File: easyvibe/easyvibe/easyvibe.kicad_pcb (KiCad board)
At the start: 2 copper layers, 111 x 54.6 mm, 80 parts, among them U1 TL062, U2 TL062, U3 TL062, U4 TL062

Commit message: some fixes
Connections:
- C2 pad 2: Net-(U1B--) -> Net-(U1B-+)
- C3 pad 2: Net-(U2B--) -> Net-(U2B-+)
- C4 pad 2: Net-(U3B--) -> Net-(U3B-+)
- C5 pad 2: Net-(U4B--) -> Net-(U4B-+)
- C6 pad 1: Net-(J_STOMP5-Pin_1) -> Net-(C6-Pad1)
- C6 pad 2: Net-(C6-Pad2) -> Net-(J_STOMP5-Pin_1)
- C8 pad 1: Net-(C8-Pad1) -> Net-(J_RATE1-Pin_1)
- LDR1 pad 1: Net-(U1B--) -> Net-(U1B-+)
- LDR2 pad 1: Net-(U2B--) -> Net-(U2B-+)
- LDR3 pad 1: Net-(U3B--) -> Net-(U3B-+)
- LDR4 pad 1: Net-(U4B--) -> Net-(U4B-+)
- R10 pad 1: Net-(U3B-+) -> Net-(U3B--)
- R11 pad 2: Net-(U4B-+) -> Net-(U4B--)
- R12 pad 1: Net-(U4B-+) -> Net-(U4B--)
- R13 pad 1: Net-(C6-Pad2) -> Net-(C6-Pad1)
- R14 pad 2: Net-(C6-Pad2) -> Net-(C6-Pad1)
- R20 pad 2: Net-(C8-Pad1) -> Net-(J_RATE1-Pin_1)
- R5 pad 2: Net-(U1B-+) -> Net-(U1B--)
- R6 pad 1: Net-(U1B-+) -> Net-(U1B--)
- R7 pad 2: Net-(U2B-+) -> Net-(U2B--)
- R8 pad 1: Net-(U2B-+) -> Net-(U2B--)
- R9 pad 2: Net-(U3B-+) -> Net-(U3B--)
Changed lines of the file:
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@@
 			(layers "*.Cu" "*.Mask")
 			(remove_unused_layers no)
-			(net "Net-(U3B-+)")
+			(net "Net-(U3B--)")
 			(pintype "passive")
 		)
@@
 			(layers "*.Cu" "*.Mask")
 			(remove_unused_layers no)
-			(net "Net-(U4B--)")
+			(net "Net-(U4B-+)")
 			(pintype "passive")
 		)
@@
 			(layers "*.Cu" "*.Mask")
 			(remove_unused_layers no)
-			(net "Net-(C8-Pad1)")
+			(net "Net-(J_RATE1-Pin_1)")
 			(pintype "passive")
 		)
@@
 			(layers "*.Cu" "*.Mask")
 			(remove_unused_layers no)
-			(net "Net-(U1B-+)")
+			(net "Net-(U1B--)")
 			(pintype "passive")
 		)
@@
 			(layers "*.Cu" "*.Mask")
 			(remove_unused_layers no)
-			(net "Net-(U2B--)")
+			(net "Net-(U2B-+)")
 			(pintype "passive")
 		)
@@
 			(layers "*.Cu" "*.Mask")
 			(remove_unused_layers no)
-			(net "Net-(U1B-+)")
+			(net "Net-(U1B--)")
 			(pintype "passive")
 		)
@@
 			(layers "*.Cu" "*.Mask")
 			(remove_unused_layers no)
-			(net "Net-(C6-Pad2)")
+			(net "Net-(C6-Pad1)")
 			(pintype "passive")
 		)
@@
 			(layers "*.Cu" "*.Mask")
 			(remove_unused_layers no)
-			(net "Net-(J_STOMP5-Pin_1)")
+			(net "Net-(C6-Pad1)")
 			(pintype "passive")
 		)
@@
 			(layers "*.Cu" "*.Mask")
 			(remove_unused_layers no)
-			(net "Net-(C6-Pad2)")
+			(net "Net-(J_STOMP5-Pin_1)")
 			(pintype "passive")
 		)
@@
 			(layers "*.Cu" "*.Mask")
 			(remove_unused_layers no)
-			(net "Net-(C6-Pad2)")
+			(net "Net-(C6-Pad1)")
 			(pintype "passive")
 		)
@@
 			(layers "*.Cu" "*.Mask")
 			(remove_unused_layers no)
-			(net "Net-(U3B-+)")
+			(net "Net-(U3B--)")
 			(pintype "passive")
 		)
@@
 			(layers "*.Cu" "*.Mask")
 			(remove_unused_layers no)
-			(net "Net-(U4B--)")
+			(net "Net-(U4B-+)")
 			(pintype "passive")
 		)
@@
 			(layers "*.Cu" "*.Mask")
 			(remove_unused_layers no)
-			(net "Net-(U1B--)")
+			(net "Net-(U1B-+)")
 			(pintype "passive")
 		)
@@
 			(layers "*.Cu" "*.Mask")
 			(remove_unused_layers no)
-			(net "Net-(U4B-+)")
+			(net "Net-(U4B--)")
 			(pintype "passive")
 		)
@@
 			(layers "*.Cu" "*.Mask")
 			(remove_unused_layers no)
-			(net "Net-(U2B--)")
+			(net "Net-(U2B-+)")
 			(pintype "passive")
 		)
@@
 			(layers "*.Cu" "*.Mask")
 			(remove_unused_layers no)
-			(net "Net-(U1B--)")
+			(net "Net-(U1B-+)")
 			(pintype "passive")
 		)
@@
 			(layers "*.Cu" "*.Mask")
 			(remove_unused_layers no)
-			(net "Net-(U4B-+)")
+			(net "Net-(U4B--)")
 			(pintype "passive")
 		)
@@
 			(remove_unused_layers no)
 			(roundrect_rratio 0.15625)
-			(net "Net-(C8-Pad1)")
+			(net "Net-(J_RATE1-Pin_1)")
 			(pintype "passive")
 		)
@@
 			(layers "*.Cu" "*.Mask")
 			(remove_unused_layers no)
-			(net "Net-(U2B-+)")
+			(net "Net-(U2B--)")
 			(pintype "passive")
 		)
@@
 			(layers "*.Cu" "*.Mask")
 			(remove_unused_layers no)
-			(net "Net-(U2B-+)")
+			(net "Net-(U2B--)")
 			(pintype "passive")
 		)
@@
 			(layers "*.Cu" "*.Mask")
 			(remove_unused_layers no)
-			(net "Net-(U3B--)")
+			(net "Net-(U3B-+)")
 			(pintype "passive")
 		)
@@
 			(layers "*.Cu" "*.Mask")
 			(remove_unused_layers no)
-			(net "Net-(U3B--)")
+			(net "Net-(U3B-+)")
 			(pintype "passive")
 		)

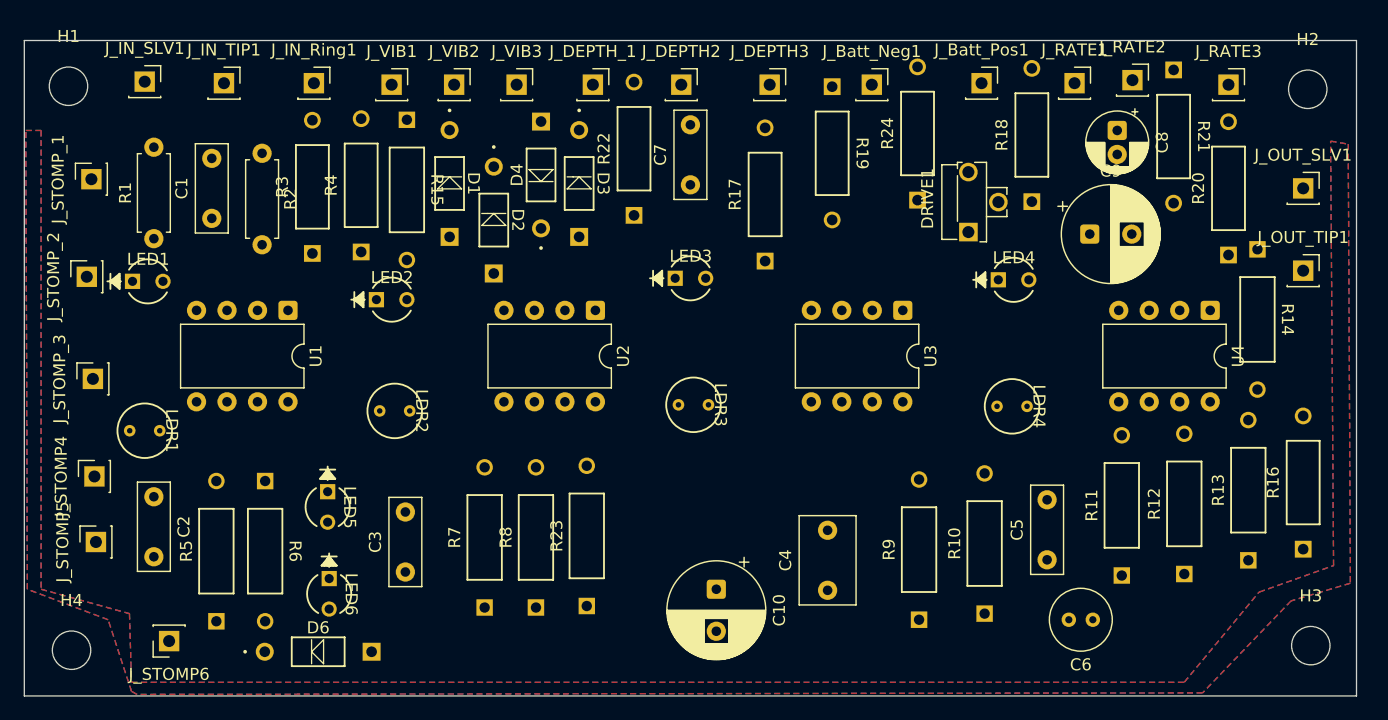
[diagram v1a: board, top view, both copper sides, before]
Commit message: more tweaks, make board slightly smaller to fit box
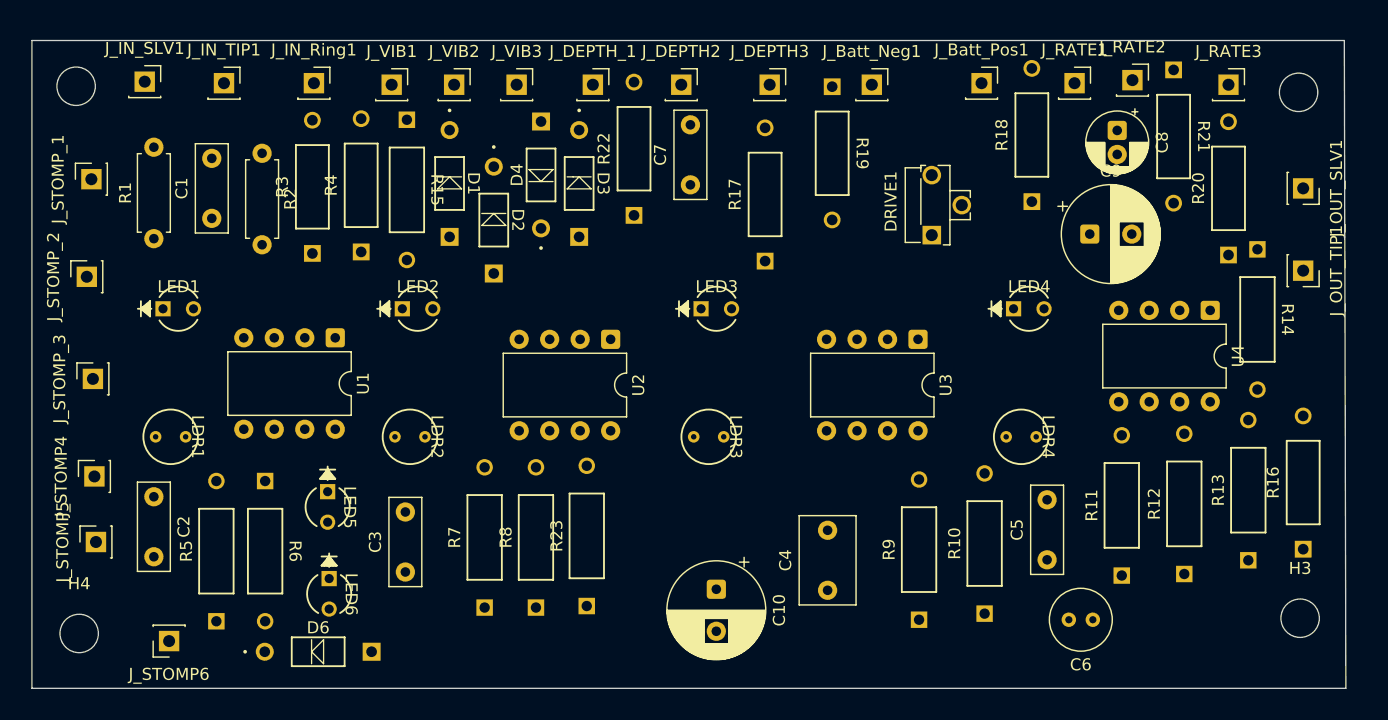
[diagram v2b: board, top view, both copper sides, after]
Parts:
- removed R24: 1K, Snapeda:RES_LR1_TYCO_TYC
- moved U1 4.55 mm to (64.3, 63.0)
- moved LED1 3.42 mm to (49.9, 60.6)
- moved LED3 3.33 mm to (94.7, 60.6)
- moved DRIVE1 3.06 mm to (114.0, 54.4)
- moved LDR3 2.95 mm to (96.6, 71.2)
- moved U2 2.73 mm to (87.2, 63.1)
- moved LED4 2.73 mm to (120.8, 60.6)
- moved U3 2.73 mm to (112.8, 63.1)
- moved LDR4 2.65 mm to (122.7, 71.2)
- moved LDR2 2.50 mm to (71.7, 71.2)
- moved H3 2.45 mm to (144.7, 86.4)
- moved LED2 2.29 mm to (69.8, 60.6)
- moved LDR1 2.22 mm to (51.8, 71.2)
- moved H4 1.53 mm to (42.9, 87.6)
- moved H2 0.80 mm to (144.5, 42.5)
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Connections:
- C10 pad 1: Net-(D6-A) -> Net-(D2-K)
- D2 pad 1: Net-(D1-A) -> Net-(D2-K)
- D2 pad 2: Net-(D2-A) -> Net-(D1-K)
- D3 pad 1: Net-(D3-K) -> Net-(D1-A)
- D3 pad 2: Net-(D1-K) -> Net-(D3-A)
- D4 pad 1: Net-(D2-A) -> Net-(D3-A)
- D4 pad 2: Net-(D3-K) -> Net-(D2-K)
- D6 pad 2: Net-(D6-A) -> Net-(D2-K)
- J_DEPTH3 pad 1: Net-(D3-K) -> Net-(D2-K)
- J_DEPTH_1 pad 1: Net-(D1-K) -> Net-(D1-A)
- LDR1 pad 2: Net-(D6-A) -> Net-(D2-K)
- LDR2 pad 2: Net-(D6-A) -> Net-(D2-K)
- LDR3 pad 2: Net-(D6-A) -> Net-(D2-K)
- LDR4 pad 2: Net-(D6-A) -> Net-(D2-K)
- R15 pad 2: Net-(D6-A) -> Net-(D2-K)
- R17 pad 2: Net-(D1-K) -> Net-(D1-A)
- R2 pad 2: Net-(D6-A) -> Net-(D2-K)
- R21 pad 2: Net-(D2-A) -> Net-(D2-K)
- R23 pad 2: Net-(D6-A) -> Net-(D2-K)
- R3 pad 2: Net-(D6-A) -> Net-(D2-K)
- U2 pad 3: Net-(D6-A) -> Net-(D2-K)
- U3 pad 3: Net-(U3A-+) -> Net-(J_DEPTH2-Pin_1)
- U4 pad 2: Net-(D2-A) -> Net-(D2-K)
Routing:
- removed copper zone on B.Cu, net GND
- removed copper zone on F.Cu, net GND
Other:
- board size 111 x 54.6 mm -> 109.5 x 54 mm
